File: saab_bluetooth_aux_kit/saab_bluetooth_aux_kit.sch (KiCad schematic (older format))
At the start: 4 parts, among them U1 CC3-0505SF-E, U2 ESP32-WROOM-DEVKIT, U3 MCP2515_MODULE, U4 UDA1334A_BREAKOUT

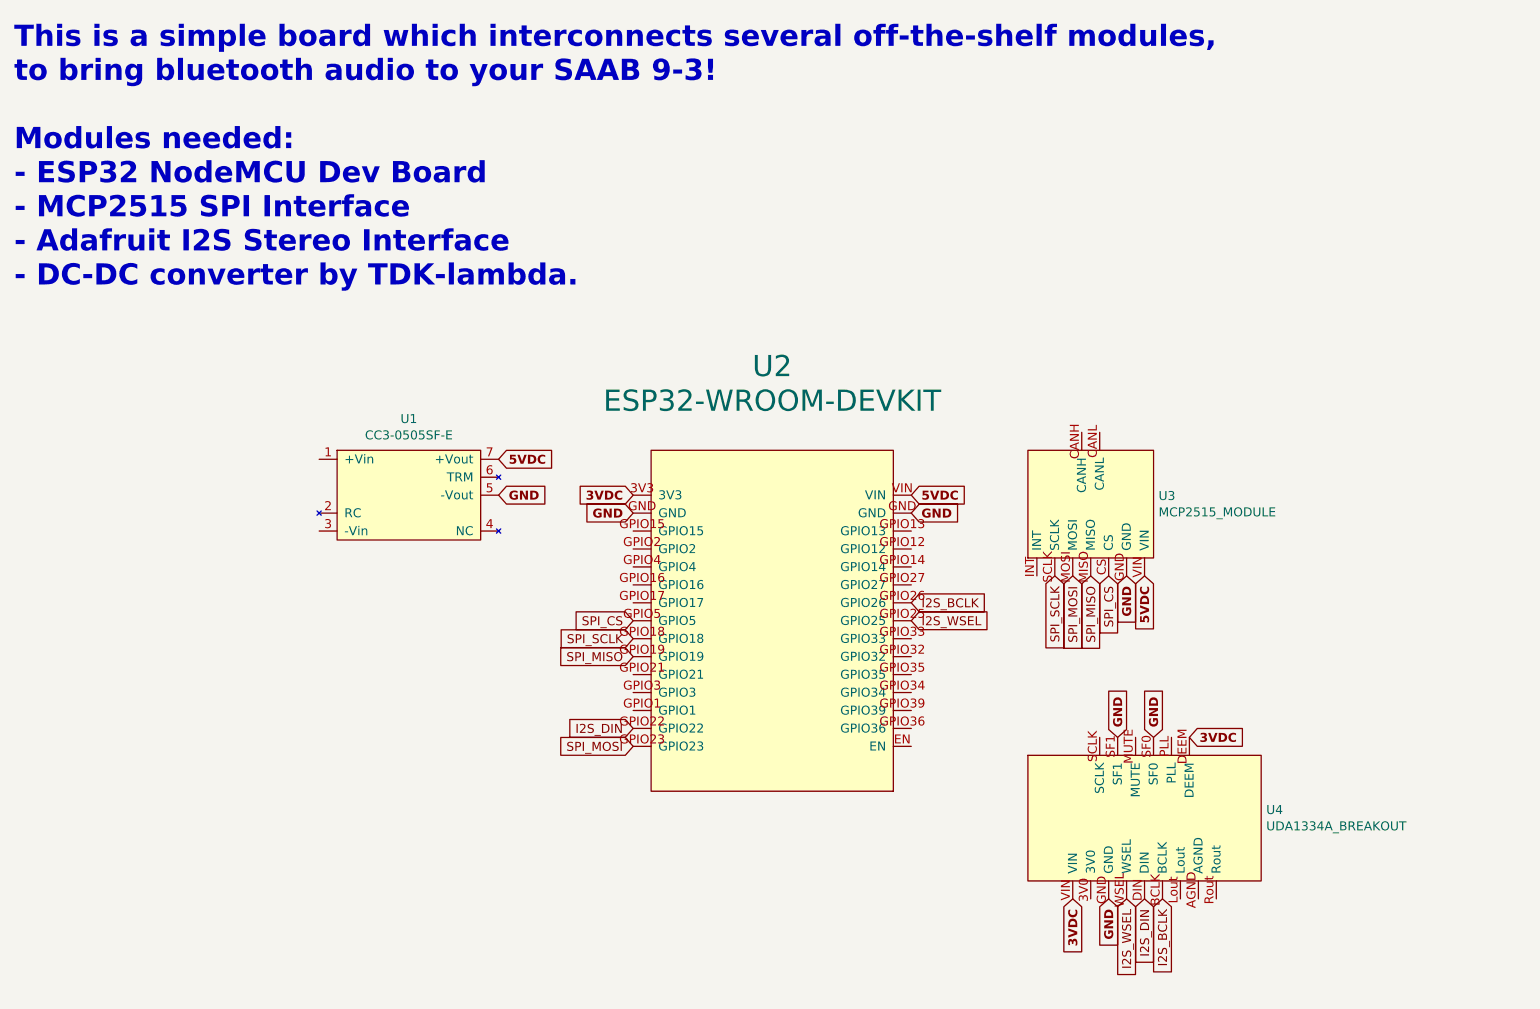
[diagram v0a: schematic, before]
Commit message: Made simple PCB
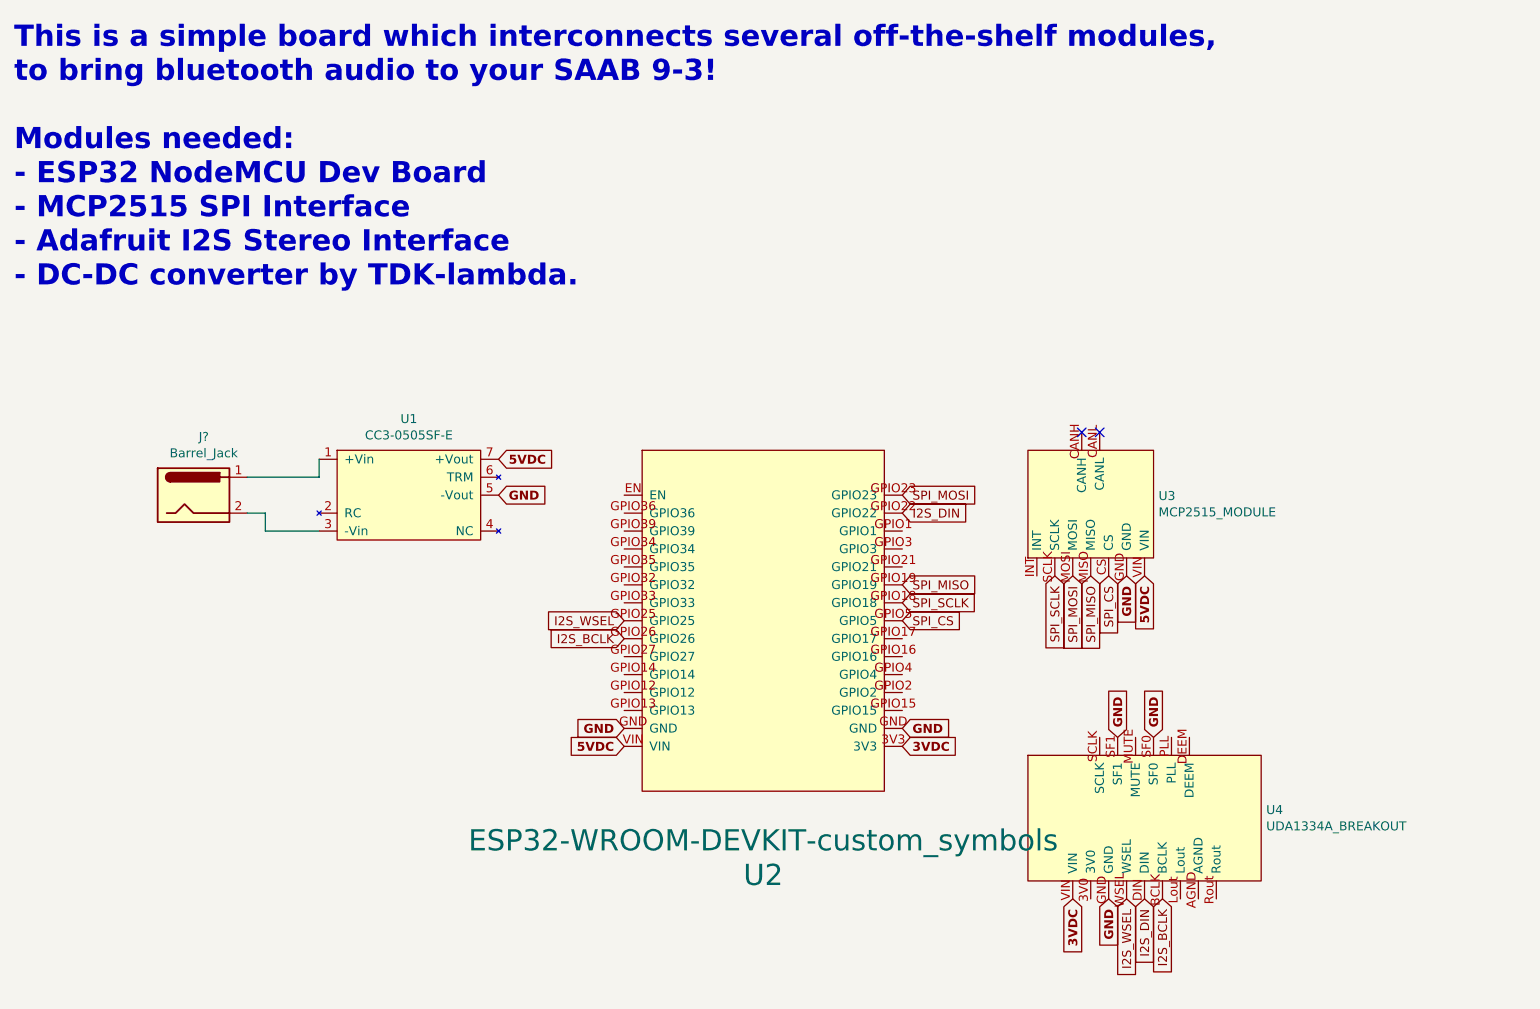
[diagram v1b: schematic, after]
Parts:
- added J?: Barrel_Jack, Connector_BarrelJack:BarrelJack_Wuerth_6941xx301002, symbol Connector:Barrel_Jack
- U2: value ESP32-WROOM-DEVKIT -> ESP32-WROOM-DEVKIT-custom_symbols
- U3: footprint (none) -> custom_footprints:MCP2515_Module
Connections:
- net 3VDC: no longer U4.DEEM
- net at U1.1 (+Vin): now also J?.1
- net at U1.3 (-Vin): now also J?.2
- no-connect marks 0 -> 2
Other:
- moved on the sheet: U2
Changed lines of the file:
@@
 L custom_symbols:ESP32-WROOM-DEVKIT U2
 U 1 1 5EA5CF06
-P 5100 4250
-F 0 "U2" H 5075 2982 118 0000 C CNN
-F 1 "ESP32-WROOM-DEVKIT" H 5075 3175 118 0000 C CNN
-F 2 "custom_footprints:ESP32-WROOM-30GPIO" H 5100 4250 118 0001 C CNN
-F 3 "" H 5100 4250 118 0001 C CNN
-	1    5100 4250
-	-1   0    0    1
+P 5100 4550
+F 0 "U2" H 5075 3282 118 0000 C CNN
+F 1 "ESP32-WROOM-DEVKIT-custom_symbols" H 5075 3475 118 0000 C CNN
+F 2 "custom_footprints:ESP32-WROOM-30GPIO" H 5100 4550 118 0001 C CNN
+F 3 "" H 5100 4550 118 0001 C CNN
+	1    5100 4550
+	1    0    0    -1
 $EndComp
 $Comp
@@
 F 0 "U3" V 6846 3272 50  0000 R CNN
 F 1 "MCP2515_MODULE" V 6755 3272 50  0000 R CNN
-F 2 "" H 6750 3750 50  0001 C CNN
+F 2 "custom_footprints:MCP2515_Module" H 6750 3750 50  0001 C CNN
 F 3 "" H 6750 3750 50  0001 C CNN
 	1    6800 3750
@@
 Text GLabel 3600 3700 2    50   Input ~ 10
 GND
-Text GLabel 5900 3800 2    50   Input ~ 10
+Text GLabel 4300 5000 0    50   Input ~ 10
 GND
-Text GLabel 5900 3700 2    50   Input ~ 10
+Text GLabel 4300 5100 0    50   Input ~ 10
 5VDC
 Text GLabel 7200 4150 3    50   Input ~ 10
@@
 Text GLabel 7100 4150 3    50   Input ~ 10
 GND
-Text GLabel 4350 3700 0    50   Input ~ 10
+Text GLabel 5850 5100 2    50   Input ~ 10
 3VDC
-Text GLabel 4350 3800 0    50   Input ~ 10
+Text GLabel 5850 5000 2    50   Input ~ 10
 GND
 Text GLabel 7000 4150 3    50   Input ~ 0
 SPI_CS
-Text GLabel 4350 4400 0    50   Input ~ 0
+Text GLabel 5850 4400 2    50   Input ~ 0
 SPI_CS
 Text GLabel 6700 4150 3    50   Input ~ 0
 SPI_SCLK
-Text GLabel 4350 4500 0    50   Input ~ 0
+Text GLabel 5850 4300 2    50   Input ~ 0
 SPI_SCLK
 Text GLabel 6900 4150 3    50   Input ~ 0
 SPI_MISO
-Text GLabel 4350 4600 0    50   Input ~ 0
+Text GLabel 5850 4200 2    50   Input ~ 0
 SPI_MISO
-Text GLabel 4350 5100 0    50   Input ~ 0
+Text GLabel 5850 3700 2    50   Input ~ 0
 SPI_MOSI
 Text GLabel 6800 4150 3    50   Input ~ 0
@@
 Text GLabel 7100 5950 3    50   Input ~ 0
 I2S_WSEL
-Text GLabel 5900 4400 2    50   Input ~ 0
+Text GLabel 4300 4400 0    50   Input ~ 0
 I2S_WSEL
 Text GLabel 7200 5950 3    50   Input ~ 0
 I2S_DIN
-Text GLabel 4350 5000 0    50   Input ~ 0
+Text GLabel 5850 3800 2    50   Input ~ 0
 I2S_DIN
 Text GLabel 7300 5950 3    50   Input ~ 0
 I2S_BCLK
-Text GLabel 5900 4300 2    50   Input ~ 0
+Text GLabel 4300 4500 0    50   Input ~ 0
 I2S_BCLK
 Text GLabel 7050 5050 1    50   Input ~ 10
@@
 Text GLabel 7250 5050 1    50   Input ~ 10
 GND
-Text GLabel 7450 5050 2    50   Input ~ 10
-3VDC
+NoConn ~ 6850 3350
+NoConn ~ 6950 3350
+$Comp
+L Connector:Barrel_Jack J?
+U 1 1 5EB35333
+P 1900 3700
+F 0 "J?" H 1957 4025 50  0000 C CNN
+F 1 "Barrel_Jack" H 1957 3934 50  0000 C CNN
+F 2 "Connector_BarrelJack:BarrelJack_Wuerth_6941xx301002" H 1950 3660 50  0001 C CNN
+F 3 "~" H 1950 3660 50  0001 C CNN
+	1    1900 3700
+	1    0    0    -1
+$EndComp
+Wire Wire Line
+	2200 3600 2600 3600
+Wire Wire Line
+	2600 3600 2600 3500
+Wire Wire Line
+	2200 3800 2300 3800
+Wire Wire Line
+	2300 3800 2300 3900
+Wire Wire Line
+	2300 3900 2600 3900
 $EndSCHEMATC
